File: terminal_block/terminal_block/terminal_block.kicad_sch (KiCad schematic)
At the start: 26 parts, among them J1 Conn_01x03, J10 Conn_01x03, J11 Conn_01x03, J12 Conn_01x03, J13 Conn_01x03, J14 Conn_01x03, J15 Conn_01x03, J16 Conn_01x03, J17 Conn_01x03, J18 Conn_01x03, J19 Conn_01x03, J2 Conn_01x03, J20 Conn_01x03, J21 Conn_01x03, J22 Conn_01x03, J23 Conn_01x03, J24 Conn_01x03, J25 Conn_01x03, J26 Conn_01x03, J3 Conn_01x03, J4 Conn_01x03, J5 Conn_01x03, J6 Conn_01x03, J7 Conn_01x03, J8 Conn_01x03, J9 Conn_01x03

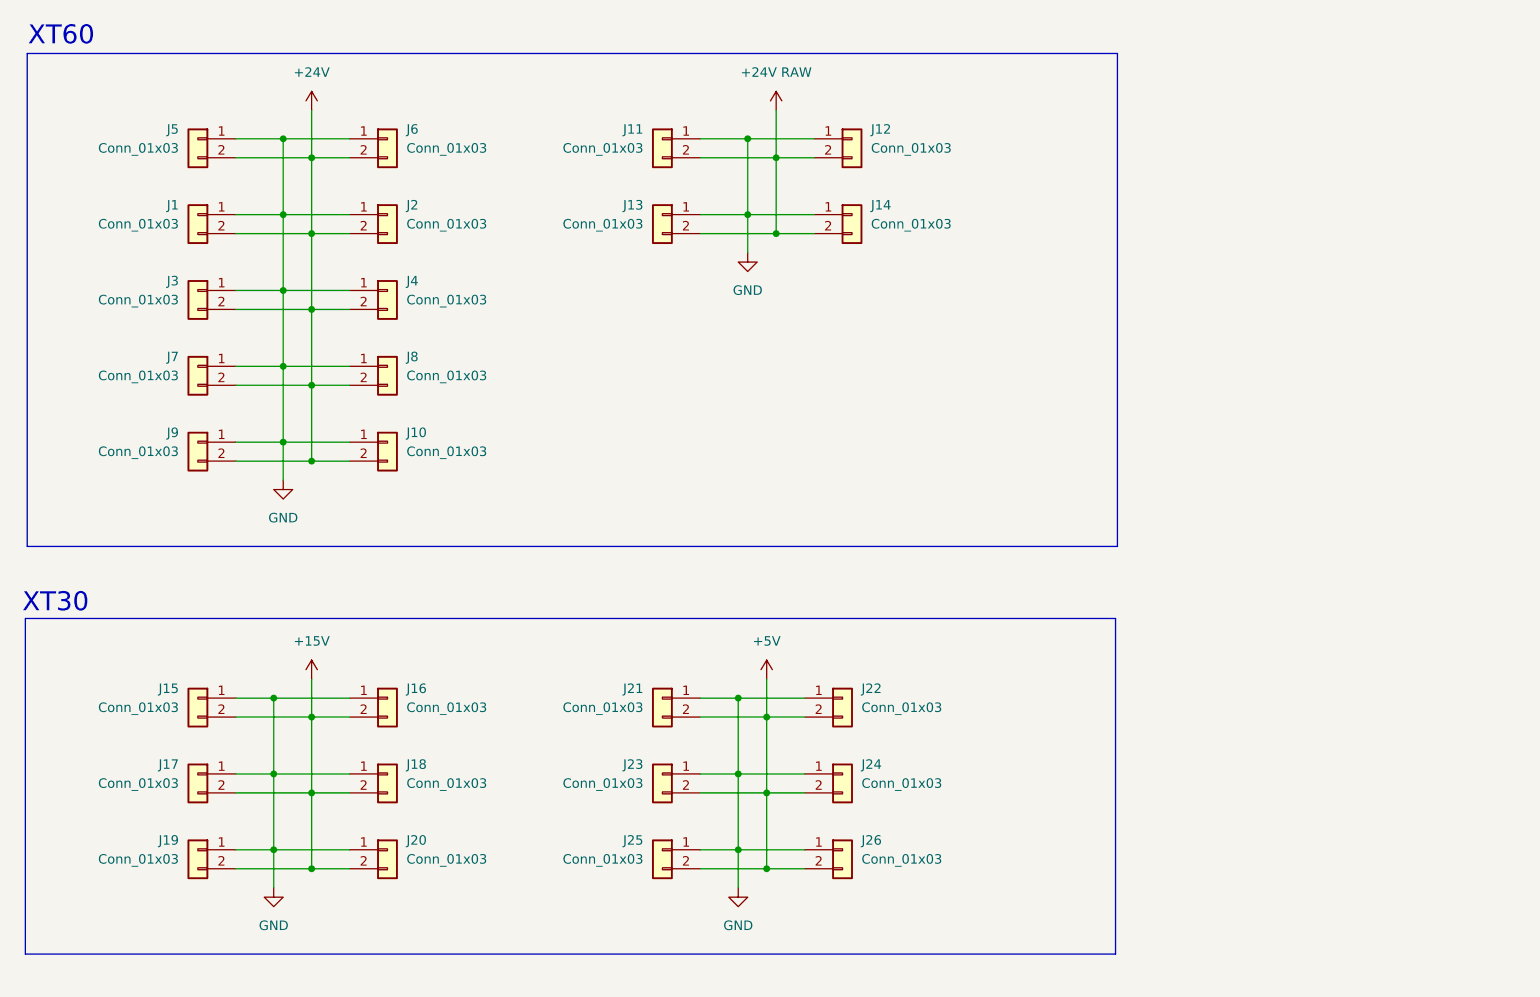
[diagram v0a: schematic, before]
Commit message: Terminal Block V3, not finished, need to check some things tomorrow
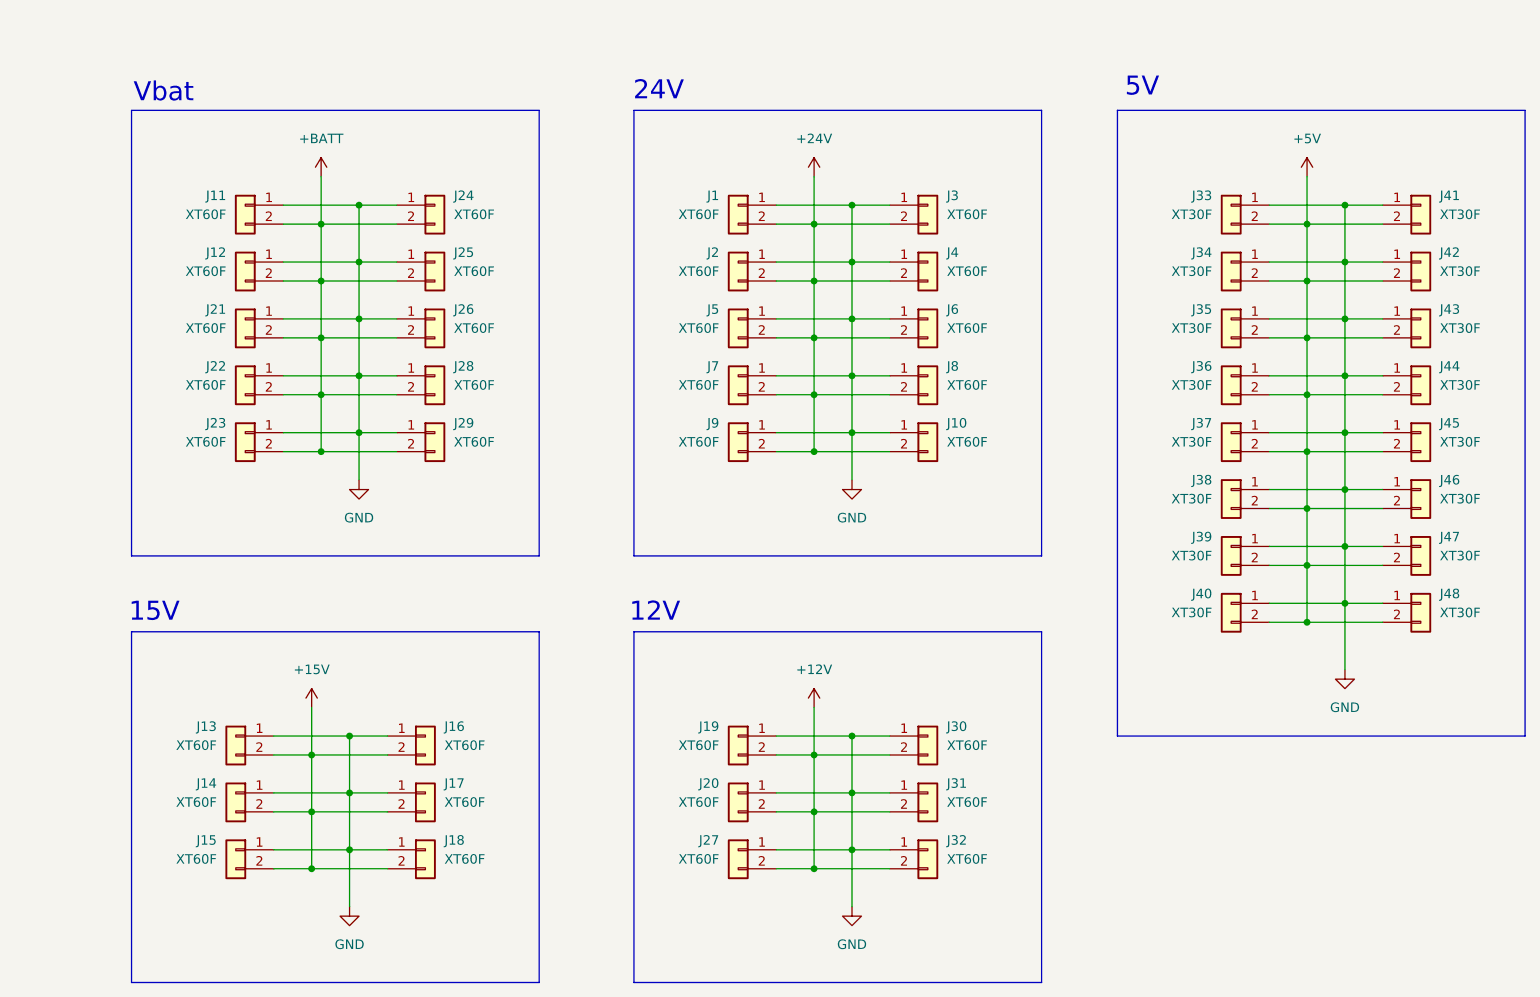
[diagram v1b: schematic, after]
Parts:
- added J27, J28, J29, J30, J31, J32: XT60F, Connector_AMASS:AMASS_XT60-F_1x02_P7.20mm_Vertical, symbol Connector_Generic:Conn_01x02
- added J33: XT30F, Connector_AMASS:AMASS_XT30UPB-F_1x02_P5.0mm_Vertical, symbol Connector_Generic:Conn_01x02
- added J34, J35, J36, J37, J38, J39, J40, J41, J42, J43, J44, J45, J46, J47, J48: XT30F, Connector_AMASS:AMASS_XT30UPB-M_1x02_P5.0mm_Vertical, symbol Connector_Generic:Conn_01x02
- J1, J10, J11, J12, J13, J14, J2, J3, J4, J5, J6, J7, J8, J9: value Conn_01x03 -> XT60F
- J15, J16, J17, J18, J19, J20, J21, J22, J23, J24, J25, J26: value Conn_01x03 -> XT60F; footprint Connector_AMASS:AMASS_XT30UPB-F_1x02_P5.0mm_Vertical -> Connector_AMASS:AMASS_XT60-F_1x02_P7.20mm_Vertical
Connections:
- net +15V: now also J13.2 (Pin_2), J14.2 (Pin_2); no longer J19.2 (Pin_2), J20.2 (Pin_2)
- net +5V: now also J33.2 (Pin_2), J34.2 (Pin_2), J35.2 (Pin_2), J36.2 (Pin_2), J37.2 (Pin_2), J38.2 (Pin_2), J39.2 (Pin_2), J40.2 (Pin_2), J41.2 (Pin_2), J42.2 (Pin_2), J43.2 (Pin_2), J44.2 (Pin_2), J45.2 (Pin_2), J46.2 (Pin_2), J47.2 (Pin_2), J48.2 (Pin_2); no longer J21.2 (Pin_2), J22.2 (Pin_2), J23.2 (Pin_2), J24.2 (Pin_2), J25.2 (Pin_2), J26.2 (Pin_2)
- net GND: now also J27.1 (Pin_1), J28.1 (Pin_1), J29.1 (Pin_1), J30.1 (Pin_1), J31.1 (Pin_1), J32.1 (Pin_1), J33.1 (Pin_1), J34.1 (Pin_1), J35.1 (Pin_1), J36.1 (Pin_1), J37.1 (Pin_1), J38.1 (Pin_1), J39.1 (Pin_1), J40.1 (Pin_1), J41.1 (Pin_1), J42.1 (Pin_1), J43.1 (Pin_1), J44.1 (Pin_1), J45.1 (Pin_1), J46.1 (Pin_1), J47.1 (Pin_1), J48.1 (Pin_1)
- net +24V RAW renamed +BATT
- net +BATT: now also J21.2 (Pin_2), J22.2 (Pin_2), J23.2 (Pin_2), J24.2 (Pin_2), J25.2 (Pin_2), J26.2 (Pin_2), J28.2 (Pin_2), J29.2 (Pin_2); no longer J13.2 (Pin_2), J14.2 (Pin_2)
- new net +12V: J19.2 (Pin_2), J20.2 (Pin_2), J27.2 (Pin_2), J30.2 (Pin_2), J31.2 (Pin_2), J32.2 (Pin_2)
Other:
- note added: "12V"
- note added: "15V"
- note added: "24V"
- note added: "5V"
- note added: "Vbat"
- note removed: "XT30"
- note removed: "XT60"
- moved on the sheet: J5, J6
